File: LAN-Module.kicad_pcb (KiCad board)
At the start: 2 copper layers, 29 x 49 mm, 70 parts, among them J1 USB_B_Micro, J2 HR911105A, J3 Conn_Left, J4 ANT, J5 Conn_Right, Q1 2N7002, Q2 2N7002, SW1 RESET, U1 ESP32-U4WDH, U2 W25Q32, U3 LV2842XLVDDCR, U4 RTL8201F, U5 CP2102N-Axx-xQFN24, Y1 40MHz ±10ppm

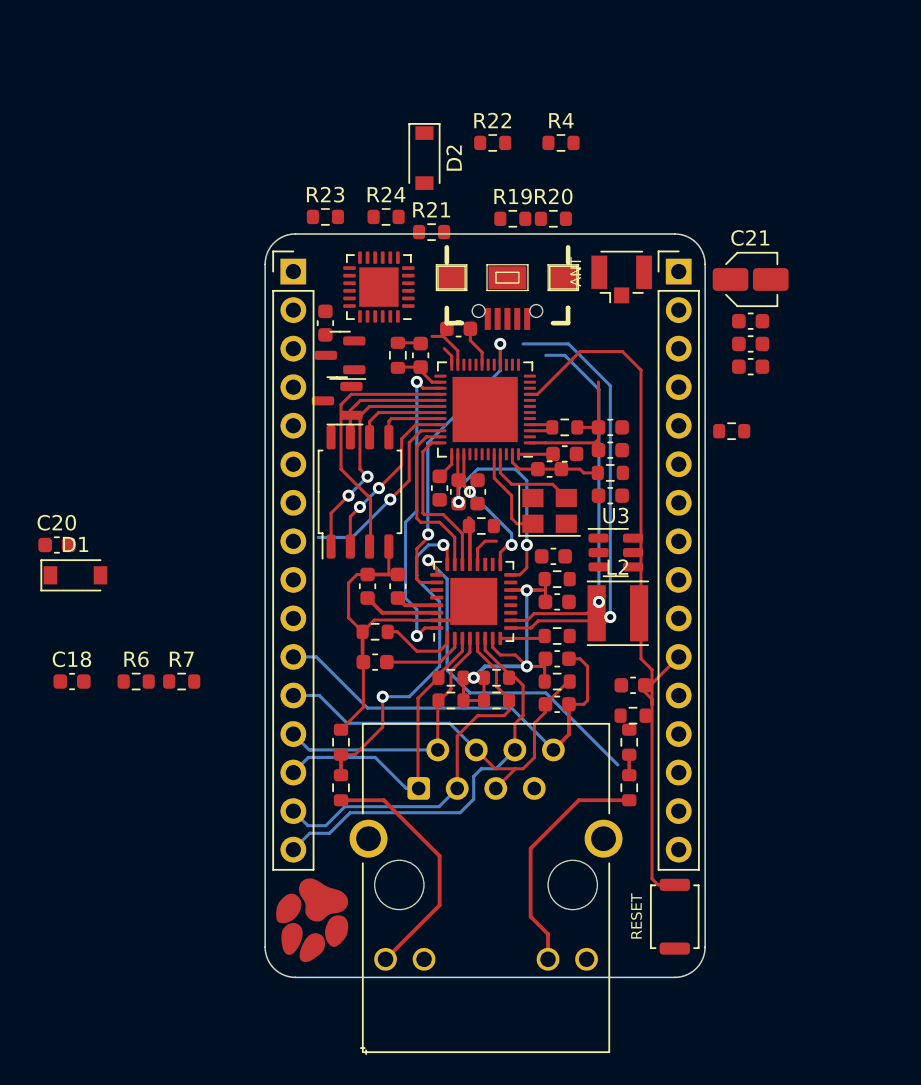
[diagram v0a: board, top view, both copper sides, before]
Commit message: Layout PCB
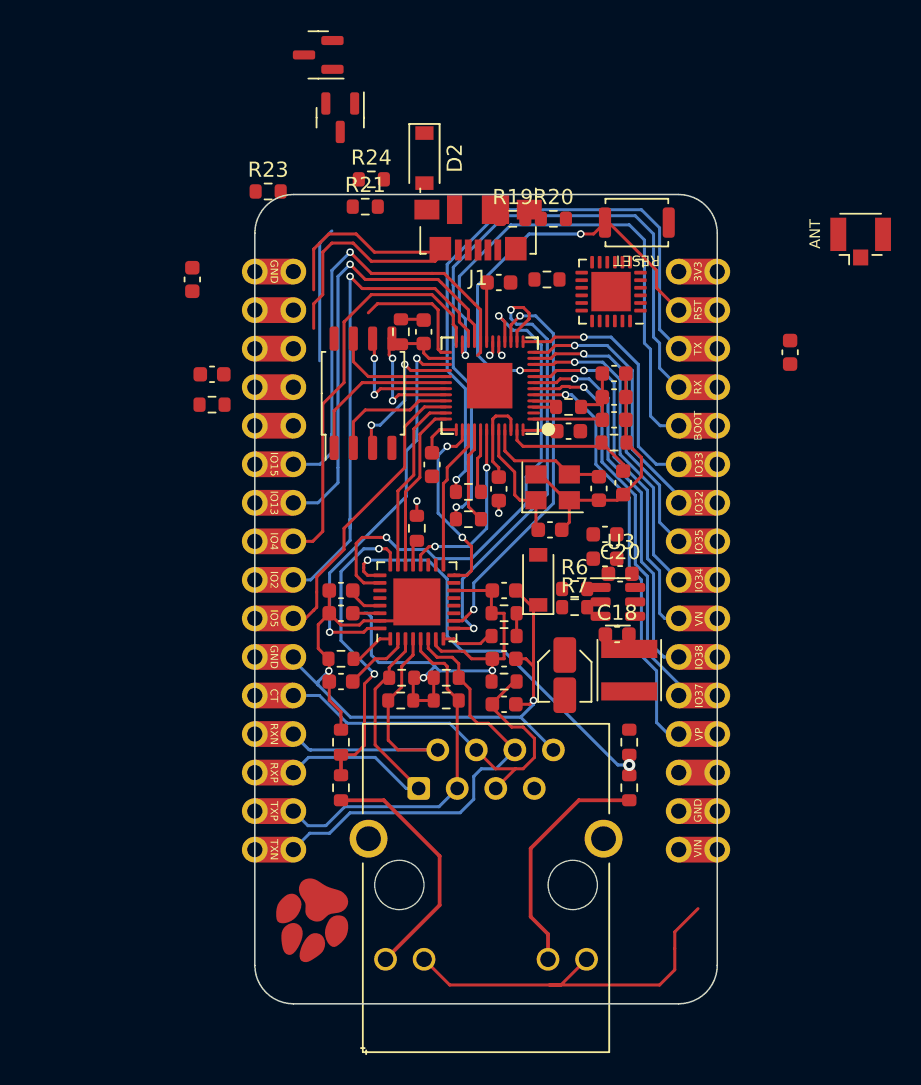
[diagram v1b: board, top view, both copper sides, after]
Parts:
- J1: footprint Visclib:USB-B-MICRO-SMD -> Connector_USB:USB_Micro-B_Molex_47346-0001
- J3, J5: footprint Connector_PinHeader_2.54mm:PinHeader_1x16_P2.54mm_Vertical -> Visclib:ProtoCastellatedHeader_1x16
- U1: footprint Package_DFN_QFN:QFN-48-1EP_6x6mm_P0.4mm_EP4.3x4.3mm -> Visclib:ESP32-REDUCED
- moved SW1 45.8 mm to (45.5, 27.2), turned to 180 degrees
- moved C20 37.2 mm to (44.4, 50.4)
- moved C18 36.1 mm to (44.2, 54.4)
- moved C10 34.5 mm to (17.5, 37.2)
- moved R1 34.5 mm to (17.5, 39.2)
- moved D1 30.5 mm to (39.0, 50.8), turned to 90 degrees
- moved R6 29.5 mm to (41.4, 51.4)
- moved C21 28.8 mm to (40.8, 57.1), turned to -90 degrees
- moved R7 26.4 mm to (41.4, 52.6)
- moved R22 24.9 mm to (34.4, 46.8)
- moved R4 23.8 mm to (34.4, 45.0)
- moved C11 23.7 mm to (55.6, 35.8)
- moved Q2 19.9 mm to (24.5, 16.2)
- moved Q1 18.7 mm to (25.9, 20.3), turned to -90 degrees
- moved C6 18.4 mm to (43.4, 49.4)
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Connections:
- J3 pad 10: /VIN -> /IO5
- J3 pad 2: /U0TXD -> /IO16
- J3 pad 3: /U0RXD -> /IO12
- J3 pad 4: /EN -> /IO14
- J3 pad 5: /BOOT -> unconnected-(J3-Pad5)
- J3 pad 6: /IO32 -> /IO13
- J3 pad 7: /IO33 -> /IO15
- J3 pad 8: /IO34 -> /IO4
- J3 pad 9: /IO35 -> /IO2
- J5 pad 10: unconnected-(J5-Pad10) -> /S_VN
- J5 pad 11: unconnected-(J5-Pad11) -> /IO38
- J5 pad 12: unconnected-(J5-Pad12) -> /IO37
- J5 pad 13: unconnected-(J5-Pad13) -> /S_VP
- J5 pad 15: unconnected-(J5-Pad15) -> GND
- J5 pad 16: GND -> /VIN
- J5 pad 2: /IO15 -> /EN
- J5 pad 3: /IO14 -> /U0TXD
- J5 pad 4: /IO13 -> /U0RXD
- J5 pad 5: /IO12 -> /BOOT
- J5 pad 6: /IO16 -> /IO33
- J5 pad 7: /IO5 -> /IO32
- J5 pad 8: /IO4 -> /IO35
- J5 pad 9: /IO2 -> /IO34
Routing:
- net GND: track 53.5 -> 121.5 mm, vias 0 -> 3
- net /U0RXD: track 0.00 -> 43.8 mm, vias 0 -> 1
- net /U0TXD: track 0.00 -> 41.3 mm, vias 0 -> 1
- net /IO2: track 0.00 -> 33.2 mm, vias 0 -> 1
- net /BOOT: track 3.01 -> 34.3 mm, vias 0 -> 1
- net /IO13: track 0.00 -> 30.8 mm, vias 0 -> 1
- net /IO15: track 0.00 -> 29.5 mm, vias 0 -> 1
- net /S_VP: track 0.00 -> 28.2 mm, vias 0 -> 1
- net /IO37: track 0.00 -> 26.3 mm, vias 0 -> 1
- net /IO4: track 1.26 -> 26.9 mm
- net /IO38: track 0.00 -> 25.1 mm, vias 0 -> 1
- net /S_VN: track 0.00 -> 23.6 mm, vias 0 -> 1
- net /IO34: track 0.00 -> 21.0 mm, vias 0 -> 1
- net /IO35: track 0.00 -> 19.3 mm, vias 0 -> 1
- net /IO32: track 0.00 -> 17.4 mm, vias 0 -> 1
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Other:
- board size 29 x 49 mm -> 30.5 x 53.3 mm
- board text added: "3V3"
- board text added: "BOOT"
- board text added: "CT"
- board text added: "GND"
- board text added: "IO13"
- board text added: "IO15"
- board text added: "IO2"
- board text added: "IO32"
- board text added: "IO33"
- board text added: "IO34"
- board text added: "IO35"
- board text added: "IO37"
- board text added: "IO38"
- board text added: "IO4"
- board text added: "IO5"
- board text added: "RST"
- board text added: "RX"
- board text added: "RXN"
- board text added: "RXP"
- board text added: "TX"
- board text added: "TXN"
- board text added: "TXP"
- board text added: "VIN"
- board text added: "VN"
- board text added: "VP"

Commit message: Final routing and placement
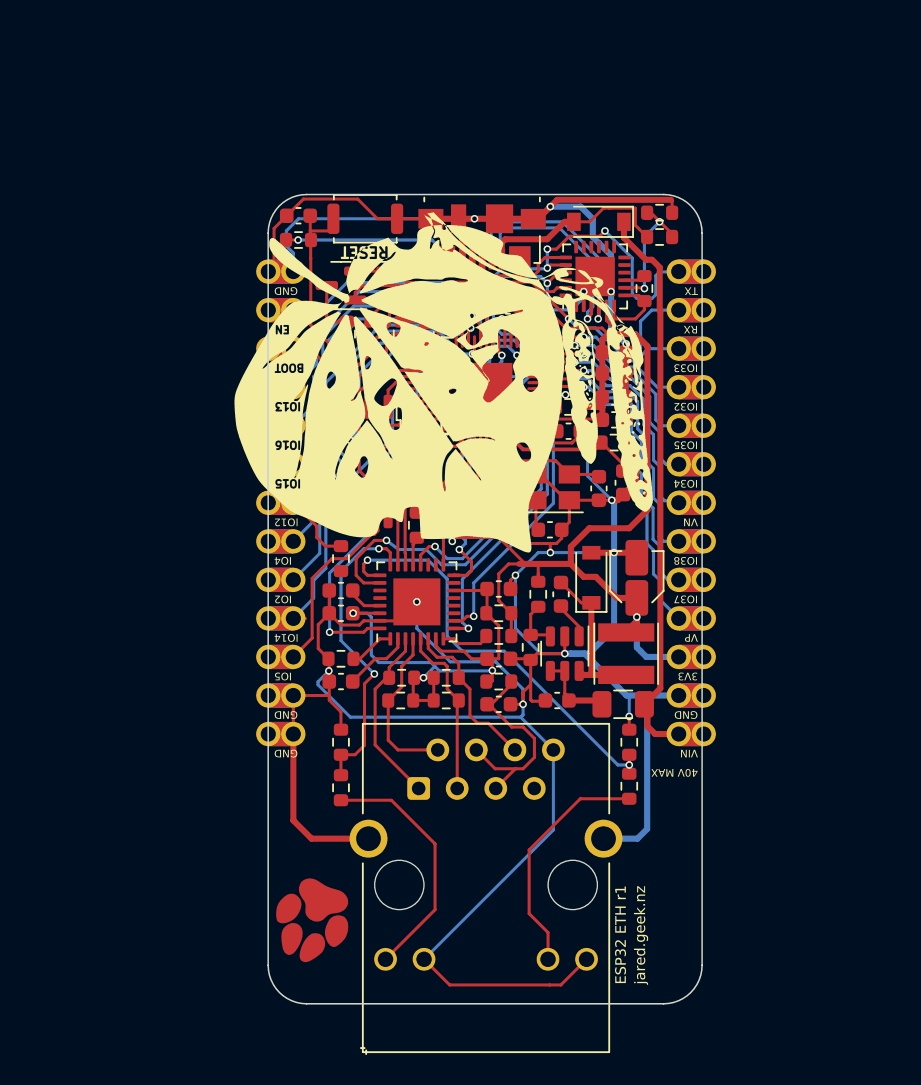
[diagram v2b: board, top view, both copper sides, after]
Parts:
- removed C27: 100n, Capacitor_SMD:C_0603_1608Metric
- removed C4: 1u, Capacitor_SMD:C_0603_1608Metric
- removed C6: 10u, Capacitor_SMD:C_0603_1608Metric
- added F1: 1A, Fuse:Fuse_1206_3216Metric, F.Cu at (44.6, 59.0)
- added J10: ProtoCastellatedHeader, Visclib:ProtoCastellatedHeader_65mil, F.Cu at (22.9, 48.3)
- added J11: ProtoCastellatedHeader, Visclib:ProtoCastellatedHeader_65mil, F.Cu at (22.9, 50.8)
- added J12: ProtoCastellatedHeader, Visclib:ProtoCastellatedHeader_65mil, F.Cu at (22.9, 53.3)
- added J13: ProtoCastellatedHeader, Visclib:ProtoCastellatedHeader_65mil, F.Cu at (22.9, 55.9)
- added J14: ProtoCastellatedHeader, Visclib:ProtoCastellatedHeader_65mil, F.Cu at (22.9, 58.4)
- added J15: ProtoCastellatedHeader, Visclib:ProtoCastellatedHeader_65mil, F.Cu at (48.3, 55.9)
- added J16: ProtoCastellatedHeader, Visclib:ProtoCastellatedHeader_65mil, F.Cu at (22.9, 61.0)
- added J17: ProtoCastellatedHeader, Visclib:ProtoCastellatedHeader_65mil, F.Cu at (48.3, 30.5)
- added J18: ProtoCastellatedHeader, Visclib:ProtoCastellatedHeader_65mil, F.Cu at (48.3, 33.0)
- added J19: ProtoCastellatedHeader, Visclib:ProtoCastellatedHeader_65mil, F.Cu at (48.3, 35.6)
- added J20: ProtoCastellatedHeader, Visclib:ProtoCastellatedHeader_65mil, F.Cu at (48.3, 38.1)
- added J21: ProtoCastellatedHeader, Visclib:ProtoCastellatedHeader_65mil, F.Cu at (48.3, 40.6)
- added J22: ProtoCastellatedHeader, Visclib:ProtoCastellatedHeader_65mil, F.Cu at (48.3, 43.2)
- added J23: ProtoCastellatedHeader, Visclib:ProtoCastellatedHeader_65mil, F.Cu at (48.3, 45.7)
- added J24: ProtoCastellatedHeader, Visclib:ProtoCastellatedHeader_65mil, F.Cu at (48.3, 48.3)
- added J25: ProtoCastellatedHeader, Visclib:ProtoCastellatedHeader_65mil, F.Cu at (48.3, 50.8)
- added J26: ProtoCastellatedHeader, Visclib:ProtoCastellatedHeader_65mil, F.Cu at (48.3, 53.3)
- added J27: ProtoCastellatedHeader, Visclib:ProtoCastellatedHeader_65mil, F.Cu at (48.3, 58.4)
- added J28: ProtoCastellatedHeader, Visclib:ProtoCastellatedHeader_65mil, F.Cu at (48.3, 61.0)
- added J6: ProtoCastellatedHeader, Visclib:ProtoCastellatedHeader_65mil, F.Cu at (22.9, 38.1)
- added J7: ProtoCastellatedHeader, Visclib:ProtoCastellatedHeader_65mil, F.Cu at (22.9, 40.6)
- added J8: ProtoCastellatedHeader, Visclib:ProtoCastellatedHeader_65mil, F.Cu at (22.9, 43.2)
- added J9: ProtoCastellatedHeader, Visclib:ProtoCastellatedHeader_65mil, F.Cu at (22.9, 45.7)
- J3: value Conn_Left -> ProtoCastellatedHeader; footprint Visclib:ProtoCastellatedHeader_1x16 -> Visclib:ProtoCastellatedHeader_65mil
- J4: value ANT -> ProtoCastellatedHeader; footprint Connector_Coaxial:U.FL_Hirose_U.FL-R-SMT-1_Vertical -> Visclib:ProtoCastellatedHeader_65mil
- J5: value Conn_Right -> ProtoCastellatedHeader; footprint Visclib:ProtoCastellatedHeader_1x16 -> Visclib:ProtoCastellatedHeader_65mil
- moved J4 37.7 mm to (22.9, 33.0), turned to 180 degrees
- moved J5 28.4 mm to (22.9, 35.6), turned to 180 degrees
- moved R5 22.9 mm to (26.0, 49.4), turned to -90 degrees
- moved R21 19.2 mm to (46.0, 31.6), turned to -90 degrees
- moved SW1 17.9 mm to (27.6, 27.0)
- moved Q2 15.3 mm to (26.0, 31.4)
- moved R1 12.3 mm to (23.2, 28.4)
- moved D2 12.2 mm to (43.0, 27.2), turned to 180 degrees
- moved C10 11.9 mm to (23.2, 26.8)
- moved Q1 11.8 mm to (30.0, 31.4), turned to 0 degrees
- moved R23 11.6 mm to (28.0, 34.6), turned to -90 degrees
- moved C11 11.6 mm to (44.0, 35.8), turned to 180 degrees
- moved R24 10.3 mm to (26.4, 34.6), turned to -90 degrees
- moved R19 9.75 mm to (47.0, 28.2), turned to 180 degrees
- moved C21 7.98 mm to (45.5, 50.7), turned to 90 degrees
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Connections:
- net Net-(C20-Pad2) renamed /SW
- net Net-(J1-Pad2) renamed /USB_N
- net Net-(J1-Pad3) renamed /USB_P
- net Net-(Q1-Pad1) renamed /RTS
- net Net-(Q1-Pad3) renamed /DTR
- net Net-(R6-Pad2) renamed /FB
- C18 pad 1: VDD -> Net-(C17-Pad1)
- D2 pad 1: VDD -> /VIN
- J4 pad 1: Net-(J4-Pad1) -> /EN
- J5 pad 1: /3V3 -> /BOOT
- L3 pad 1: VDD -> +3V3
- R10 pad 1: VDD -> +3V3
- R9 pad 1: VDD -> +3V3
- U1 pad 2: Net-(J4-Pad1) -> unconnected-(U1-Pad2)
- U3 pad 4: VDD -> Net-(C17-Pad1)
- U3 pad 5: VDD -> Net-(C17-Pad1)
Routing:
- net GND: track 121.5 -> 312.5 mm, vias 3 -> 24
- net +3V3: track 22.2 -> 128.5 mm, vias 0 -> 7
- net /VIN: track 0.00 -> 36.2 mm
- net /IO14: track 0.98 -> 32.2 mm
- net /IO12: track 0.98 -> 28.6 mm, vias 1 -> 2
- net /MDI1_N: track 29.1 -> 10.9 mm
- net /BOOT: track 34.3 -> 16.6 mm, vias 1 -> 0
- net /USB_P: track 0.00 -> 15.8 mm, vias 0 -> 2
- net /USB_N: track 0.00 -> 15.3 mm, vias 0 -> 2
- net /DTR: track 0.00 -> 15.0 mm
- net /RTS: track 0.00 -> 14.8 mm
- net /MDI0_CT: track 27.8 -> 14.2 mm
- net VBUS: track 0.00 -> 13.1 mm
- net /SDD0: track 0.00 -> 13.0 mm, vias 0 -> 2
- net /IO13: track 30.8 -> 18.1 mm
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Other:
- board size 30.5 x 53.3 mm -> 28.6 x 53.3 mm
- board text added: "40V MAX"
- board text added: "ESP32 ETH r1"
- board text added: "ETHERNET"
- board text added: "GPIO"
- board text added: "IO12"
- board text added: "IO14"
- board text added: "LNA ADC"
- board text added: "UART"
- board text added: "USB-UART"
- board text added: "jared.geek.nz"
- board text removed: "BOOT"
- board text removed: "CT"
- board text removed: "IO13"
- board text removed: "IO15"
- board text removed: "RST"
- board text removed: "RXN"
- board text removed: "RXP"
- board text removed: "TXN"
- board text removed: "TXP"
